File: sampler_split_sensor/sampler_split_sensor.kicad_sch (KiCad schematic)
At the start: 94 parts, among them J1 TSW-120-20-S-D-LL, J2 Conn_01x32_Pin, J3 Conn_01x32_Pin, U1 Teensy4.1, U10 DRV5055A1xLPGxQ1, U11 DRV5055A1xLPGxQ1, U12 DRV5055A1xLPGxQ1, U13 DRV5055A1xLPGxQ1, U14 DRV5055A1xLPGxQ1, U15 DRV5055A1xLPGxQ1, U16 DRV5055A1xLPGxQ1, U17 DRV5055A1xLPGxQ1, U18 DRV5055A1xLPGxQ1, U19 DRV5055A1xLPGxQ1, U2 DRV5055A1xLPGxQ1, U3 DRV5055A1xLPGxQ1, U4 DRV5055A1xLPGxQ1, U5 DRV5055A1xLPGxQ1, U6 DRV5055A1xLPGxQ1, U7 DRV5055A1xLPGxQ1, U8 DRV5055A1xLPGxQ1, U9 DRV5055A1xLPGxQ1

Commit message: add split sensor board for breakaway
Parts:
- added J4, J5: Conn_01x32_Pin, mine:Conn_1x32_SMD, symbol Connector:Conn_01x32_Pin
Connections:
- net GND: now also J4.1 (Pin_1), J4.6 (Pin_6), J5.27 (Pin_27), J5.32 (Pin_32)
- net at BOARDSEL_CMP1.14 (VCC), BOARDSEL_ENABLE1.14 (VCC), DG452_0.12 (V_L)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: now also J4.3 (Pin_3), J4.4 (Pin_4), J5.29 (Pin_29), J5.30 (Pin_30)
- net at JP19.2 (B), JP54.1 (A), U8.3 (OUT): now also J4.26 (Pin_26), J5.7 (Pin_7)
- net at J1.28, JP21.1 (A), JPE14.1 (A)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: no longer DG452_3.7 (D_4), J2.19 (Pin_19), J3.19 (Pin_19), JPE14.2 (B)
- net at J1.04, JP9.1 (A), JPE02.1 (A)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: no longer DG452_0.7 (D_4), J2.31 (Pin_31), J3.31 (Pin_31), JPE02.2 (B)
- net at JP10.2 (B), JP24.2 (B), JP63.1 (A)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: now also J4.17 (Pin_17), J5.16 (Pin_16)
- net at DG452_3.10 (D_3), J2.17 (Pin_17), J3.17 (Pin_17)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: no longer J1.32, JP45.1 (A), JPE16.1 (A), U1.38 (16_A2_RX4_SCL1)
- net at DG452_3.14 (S_2), J2.18 (Pin_18), J3.18 (Pin_18)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: no longer J1.30, JP22.1 (A), JPE15.1 (A), U1.39 (17_A3_TX4_SDA1)
- net at DG452_3.3 (S_1), J2.20 (Pin_20), J3.20 (Pin_20)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: no longer J1.26, JP20.1 (A), JPE13.1 (A), U1.41 (19_A5_SCL)
- net at JP16.2 (B), JP57.1 (A), U11.3 (OUT): now also J4.23 (Pin_23), J5.10 (Pin_10)
- net at J1.12, JP13.1 (A), JPE06.1 (A)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: no longer DG452_1.7 (D_4), J2.27 (Pin_27), J3.27 (Pin_27), JPE06.2 (B)
- net at J1.22, JP18.1 (A), JPE11.1 (A)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: no longer DG452_2.14 (S_2), J2.22 (Pin_22), J3.22 (Pin_22), JPE11.2 (B)
- net at J1.34, JP46.1 (A), JPE17.1 (A)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: no longer DG45_4.3 (S_1), J2.16 (Pin_16), J3.16 (Pin_16), JPE17.2 (B)
- net at JP46.2 (B), JP49.1 (A), U3.3 (OUT): now also J4.31 (Pin_31), J5.2 (Pin_2)
- net at J1.36, JP47.1 (A), JPE18.1 (A)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: no longer DG45_4.7 (D_4), J2.15 (Pin_15), J3.15 (Pin_15), JPE18.2 (B)
- net at JP11.2 (B), JP62.1 (A), JP7.2 (B)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: now also J4.18 (Pin_18), J5.15 (Pin_15)
- net at JP45.2 (B), JP50.1 (A), U4.3 (OUT): now also J4.30 (Pin_30), J5.3 (Pin_3)
- net at JP12.2 (B), JP6.2 (B), JP61.1 (A)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: now also J4.19 (Pin_19), J5.14 (Pin_14)
- net at JP21.2 (B), JP52.1 (A), U6.3 (OUT): now also J4.28 (Pin_28), J5.5 (Pin_5)
- net at J1.10, JP12.1 (A), JPE05.1 (A)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: no longer DG452_1.3 (S_1), J2.28 (Pin_28), J3.28 (Pin_28), JPE05.2 (B)
- net at DG452_1.10 (D_3), J2.25 (Pin_25), J3.25 (Pin_25)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: no longer J1.16, JP15.1 (A), JPE08.1 (A), U1.30 (38_CS1_IN1)
- net at DG452_1.14 (S_2), J2.26 (Pin_26), J3.26 (Pin_26)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: no longer J1.14, JP14.1 (A), JPE07.1 (A), U1.31 (39_MISO1_OUT1A)
- net at JP25.2 (B), JP64.1 (A), JP9.2 (B)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: now also J4.16 (Pin_16), J5.17 (Pin_17)
- net at JP20.2 (B), JP53.1 (A), U7.3 (OUT): now also J4.27 (Pin_27), J5.6 (Pin_6)
- net at JP15.2 (B), JP58.1 (A), U12.3 (OUT): now also J4.22 (Pin_22), J5.11 (Pin_11)
- net at J1.20, JP17.1 (A), JPE10.1 (A)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: no longer DG452_2.7 (D_4), J2.23 (Pin_23), J3.23 (Pin_23), JPE10.2 (B)
- net at JP18.2 (B), JP55.1 (A), U9.3 (OUT): now also J4.25 (Pin_25), J5.8 (Pin_8)
- net at J1.08, JP11.1 (A), JPE04.1 (A)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: no longer DG452_0.10 (D_3), J2.29 (Pin_29), J3.29 (Pin_29), JPE04.2 (B)
- net at JP17.2 (B), JP56.1 (A), U10.3 (OUT): now also J4.24 (Pin_24), J5.9 (Pin_9)
- net at J1.06, JP10.1 (A), JPE03.1 (A)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: no longer DG452_0.14 (S_2), J2.30 (Pin_30), J3.30 (Pin_30), JPE03.2 (B)
- net at JP47.2 (B), JP48.1 (A), U2.3 (OUT): now also J4.32 (Pin_32), J5.1 (Pin_1)
- net at JP22.2 (B), JP51.1 (A), U5.3 (OUT): now also J4.29 (Pin_29), J5.4 (Pin_4)
- net at J1.24, JP19.1 (A), JPE12.1 (A)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: no longer DG452_2.10 (D_3), J2.21 (Pin_21), J3.21 (Pin_21), JPE12.2 (B)
- net at JP14.2 (B), JP59.1 (A), U13.3 (OUT): now also J4.21 (Pin_21), J5.12 (Pin_12)
- net at JP13.2 (B), JP5.2 (B), JP60.1 (A)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: now also J4.20 (Pin_20), J5.13 (Pin_13)
- net at J1.02, JP8.1 (A), JPE01.1 (A)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: no longer DG452_0.3 (S_1), J2.32 (Pin_32), J3.32 (Pin_32), JPE01.2 (B)
- net at JP26.2 (B), JP65.1 (A), JP8.2 (B)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: now also J4.15 (Pin_15), J5.18 (Pin_18)
- net at DG452_2.3 (S_1), J2.24 (Pin_24), J3.24 (Pin_24)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: no longer J1.18, JP16.1 (A), JPE09.1 (A), U1.45 (23_A9_CRX1_MCLK1)
- new net: DG452_3.7 (D_4), J2.19 (Pin_19), J3.19 (Pin_19), JPE14.2 (B)
- new net: DG452_0.7 (D_4), J2.31 (Pin_31), J3.31 (Pin_31), JPE02.2 (B)
- new net: DG452_1.7 (D_4), J2.27 (Pin_27), J3.27 (Pin_27), JPE06.2 (B)
- new net: DG452_2.14 (S_2), J2.22 (Pin_22), J3.22 (Pin_22), JPE11.2 (B)
- new net: DG45_4.7 (D_4), J2.15 (Pin_15), J3.15 (Pin_15), JPE18.2 (B)
- new net: DG452_1.3 (S_1), J2.28 (Pin_28), J3.28 (Pin_28), JPE05.2 (B)
- new net: J1.32, JP45.1 (A), JPE16.1 (A), U1.38 (16_A2_RX4_SCL1)
- new net: J1.26, JP20.1 (A), JPE13.1 (A), U1.41 (19_A5_SCL)
- new net: DG452_2.7 (D_4), J2.23 (Pin_23), J3.23 (Pin_23), JPE10.2 (B)
- new net: DG452_0.14 (S_2), J2.30 (Pin_30), J3.30 (Pin_30), JPE03.2 (B)
- new net: J1.30, JP22.1 (A), JPE15.1 (A), U1.39 (17_A3_TX4_SDA1)
- new net: DG452_2.10 (D_3), J2.21 (Pin_21), J3.21 (Pin_21), JPE12.2 (B)
- new net: J1.14, JP14.1 (A), JPE07.1 (A), U1.31 (39_MISO1_OUT1A)
- new net: J1.16, JP15.1 (A), JPE08.1 (A), U1.30 (38_CS1_IN1)
- new net: DG45_4.3 (S_1), J2.16 (Pin_16), J3.16 (Pin_16), JPE17.2 (B)
- new net: DG452_0.10 (D_3), J2.29 (Pin_29), J3.29 (Pin_29), JPE04.2 (B)
- new net: DG452_0.3 (S_1), J2.32 (Pin_32), J3.32 (Pin_32), JPE01.2 (B)
- new net: J1.18, JP16.1 (A), JPE09.1 (A), U1.45 (23_A9_CRX1_MCLK1)
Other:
- moved on the sheet: BOARDSEL_CMP1, BOARDSEL_ENABLE1, DG452_0, DG452_1, DG452_2, DG452_3, DG45_4, J1, J2, J3, JP1, JP2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

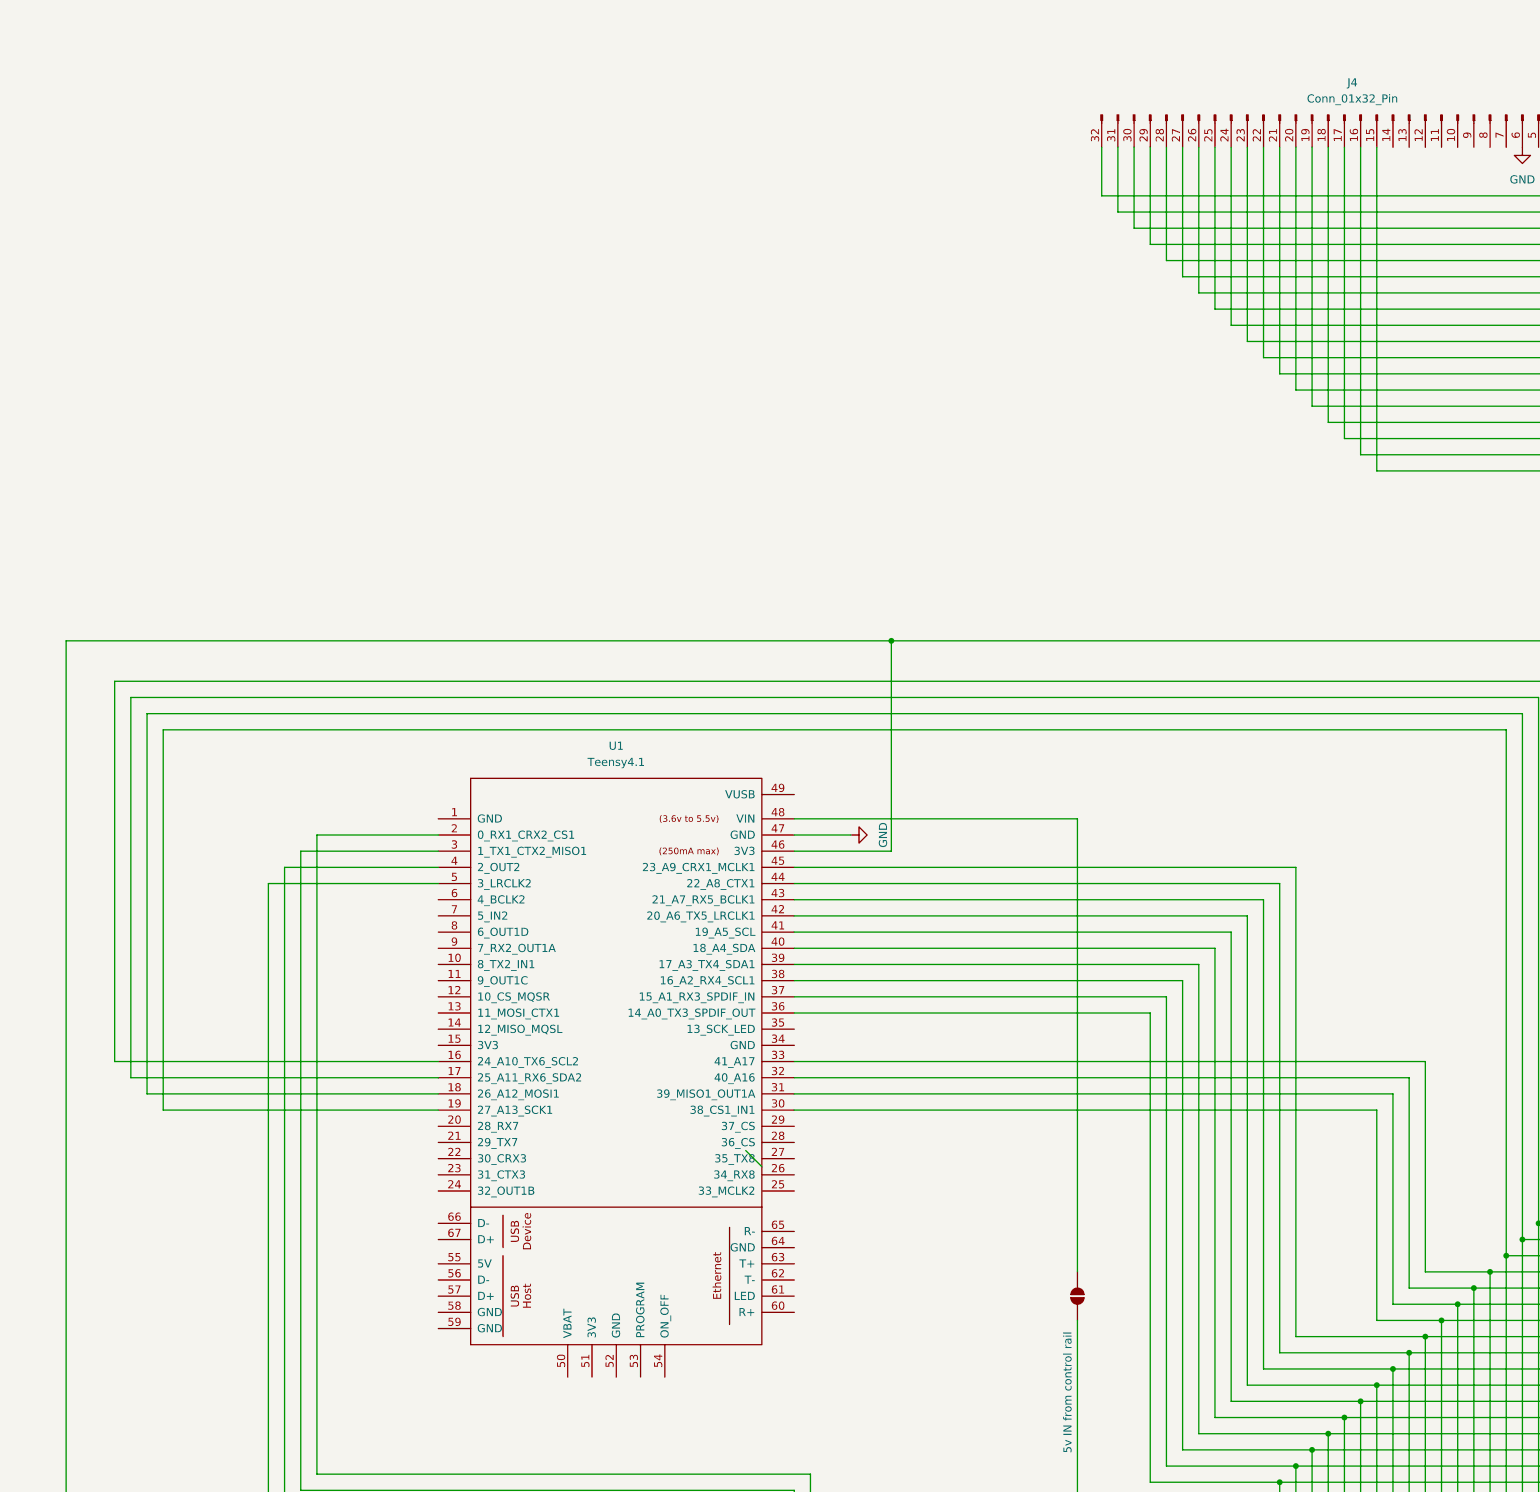
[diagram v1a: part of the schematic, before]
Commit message: Boards v3
Signed-off-by: Sawyer Bergeron <sawyerbergeron@gmail.com>
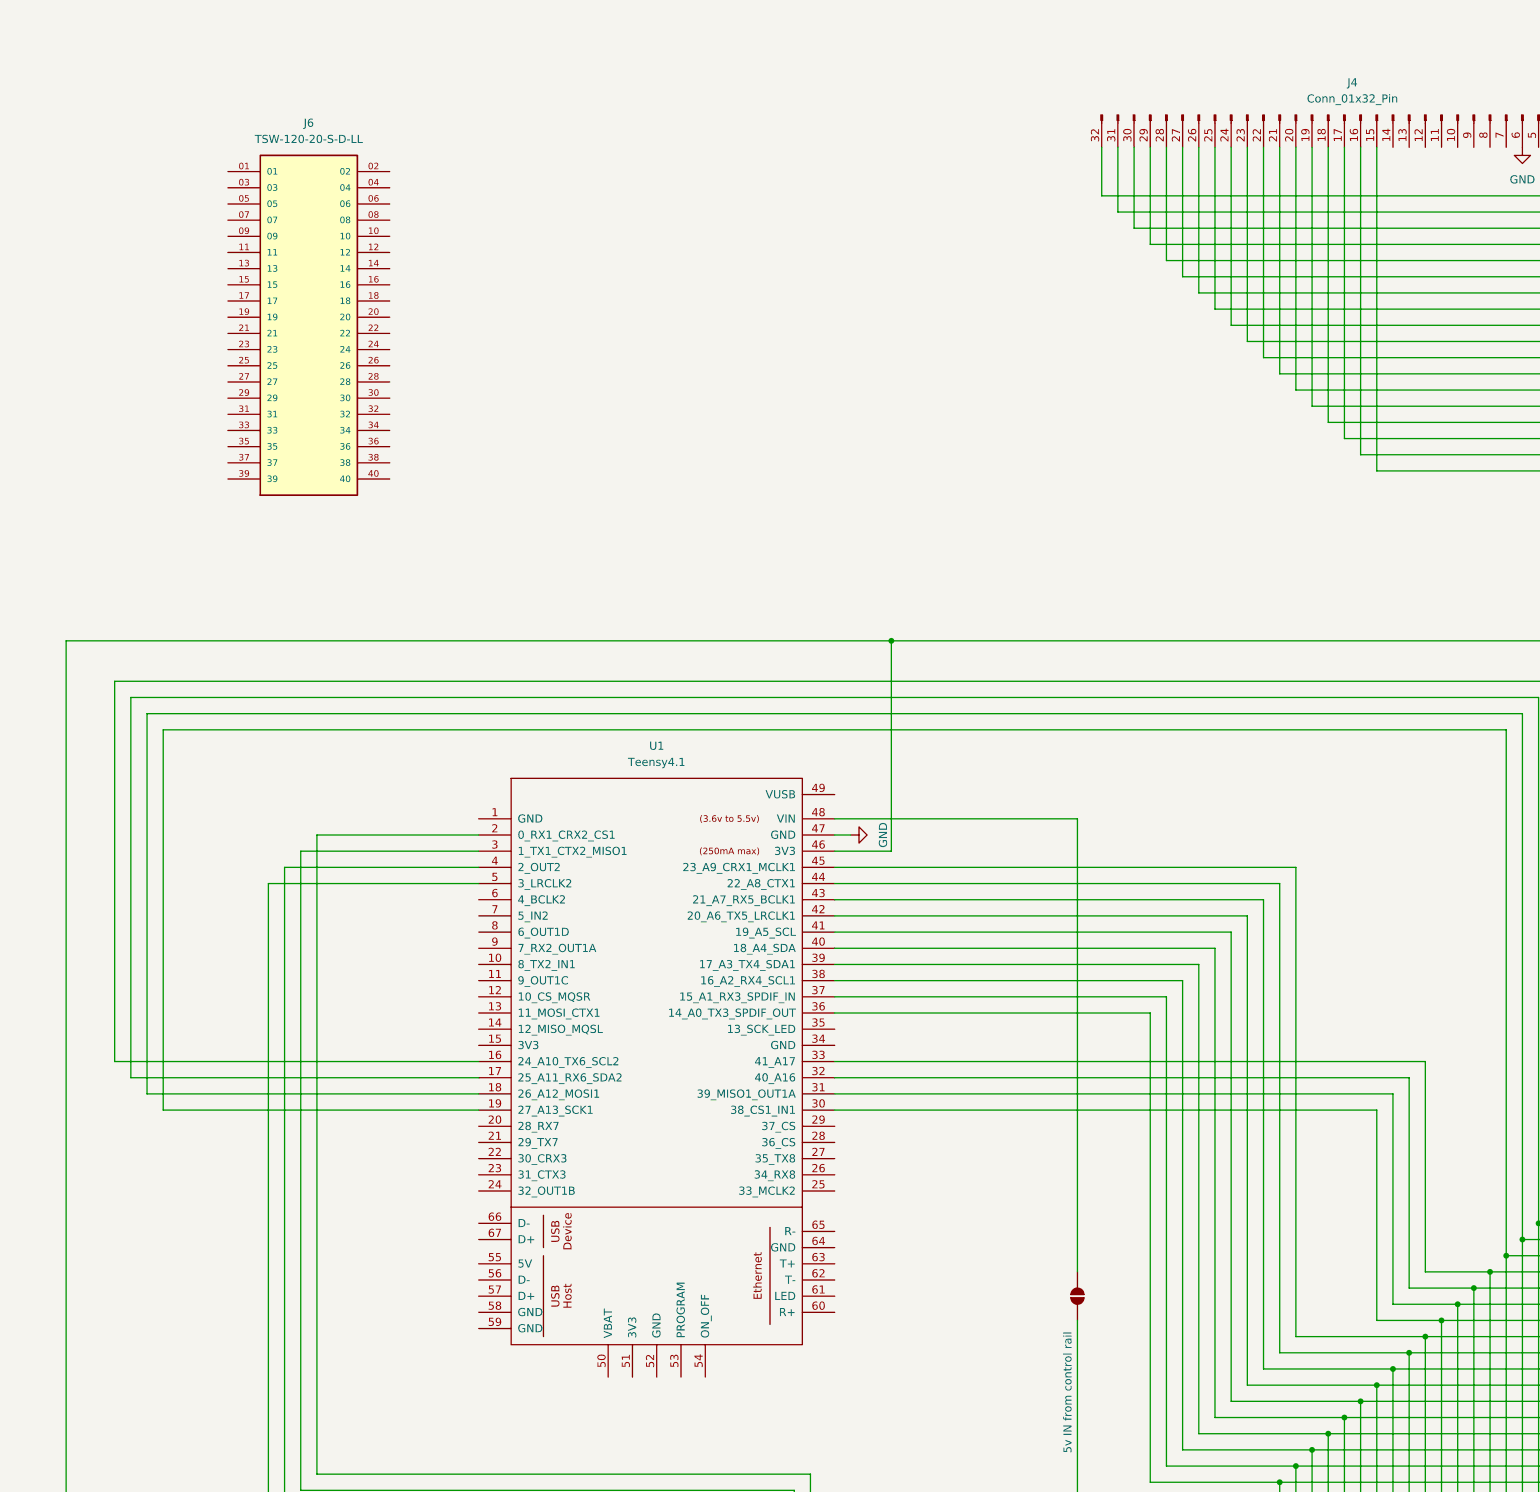
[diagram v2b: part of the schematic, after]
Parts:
- added J6: TSW-120-20-S-D-LL, mine:SAMTEC_TSW-120-20-S-D-LL, symbol mine:TSW-120-20-S-D-LL
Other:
- moved on the sheet: U1
